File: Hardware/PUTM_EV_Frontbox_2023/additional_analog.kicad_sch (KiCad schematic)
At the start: 11 parts, among them U15 DNP

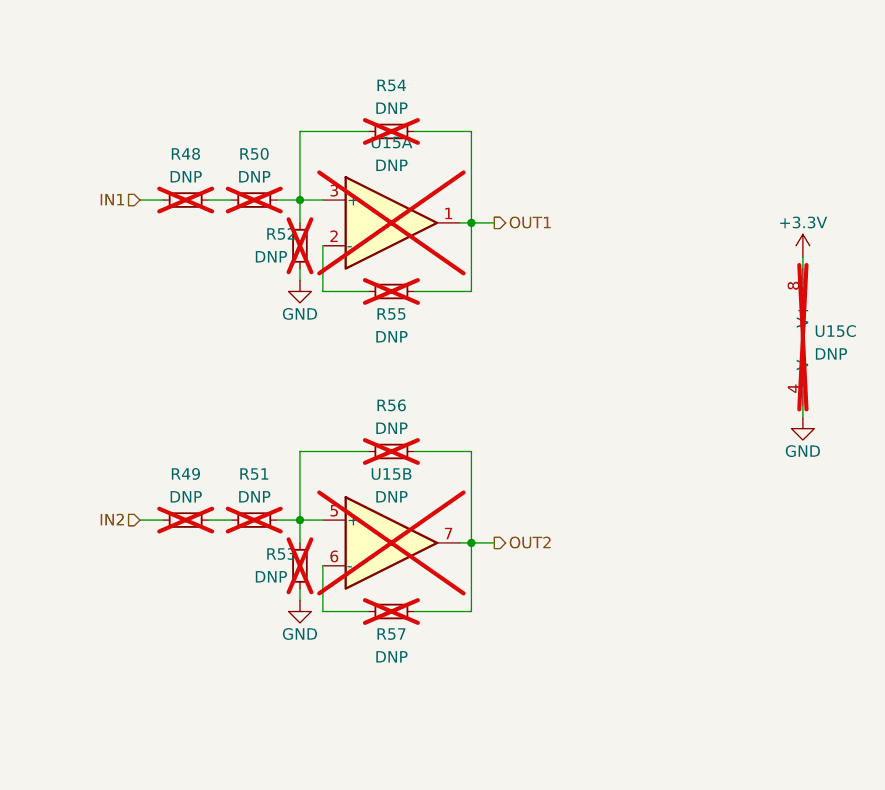
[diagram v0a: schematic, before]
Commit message: Fixed all issues
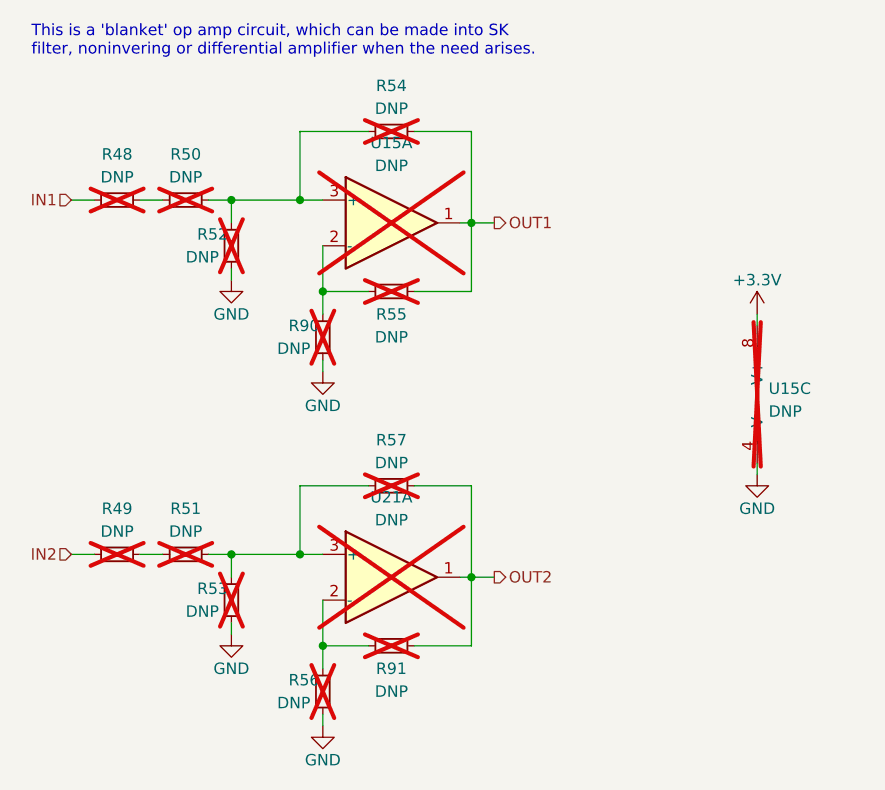
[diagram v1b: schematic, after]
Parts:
- removed unit 2 of U15
- added R90, R91: DNP, symbol Device:R_Small
- added U21: DNP, symbol Amplifier_Operational:TLV9062
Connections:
- net GND: now also R56.2, R90.2
- net OUT2: now also R57.1, R91.2, U21.1; no longer R56.1, R57.2
- net at R55.1, U15.2 (-): now also R90.1
- net at R51.2, R53.1: now also R57.2, U21.3 (+); no longer R56.2
- new net: R56.1, R91.1, U21.2 (-)
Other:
- note added: "This is a 'blanket' op amp circuit, which can be made into SK filter, noninvering or differential amplifier when the need arises."
- moved on the sheet: R48, R50, R52, U15C
